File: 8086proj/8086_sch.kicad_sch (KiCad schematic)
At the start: 1 part, among them U1 8086_Min_Mode

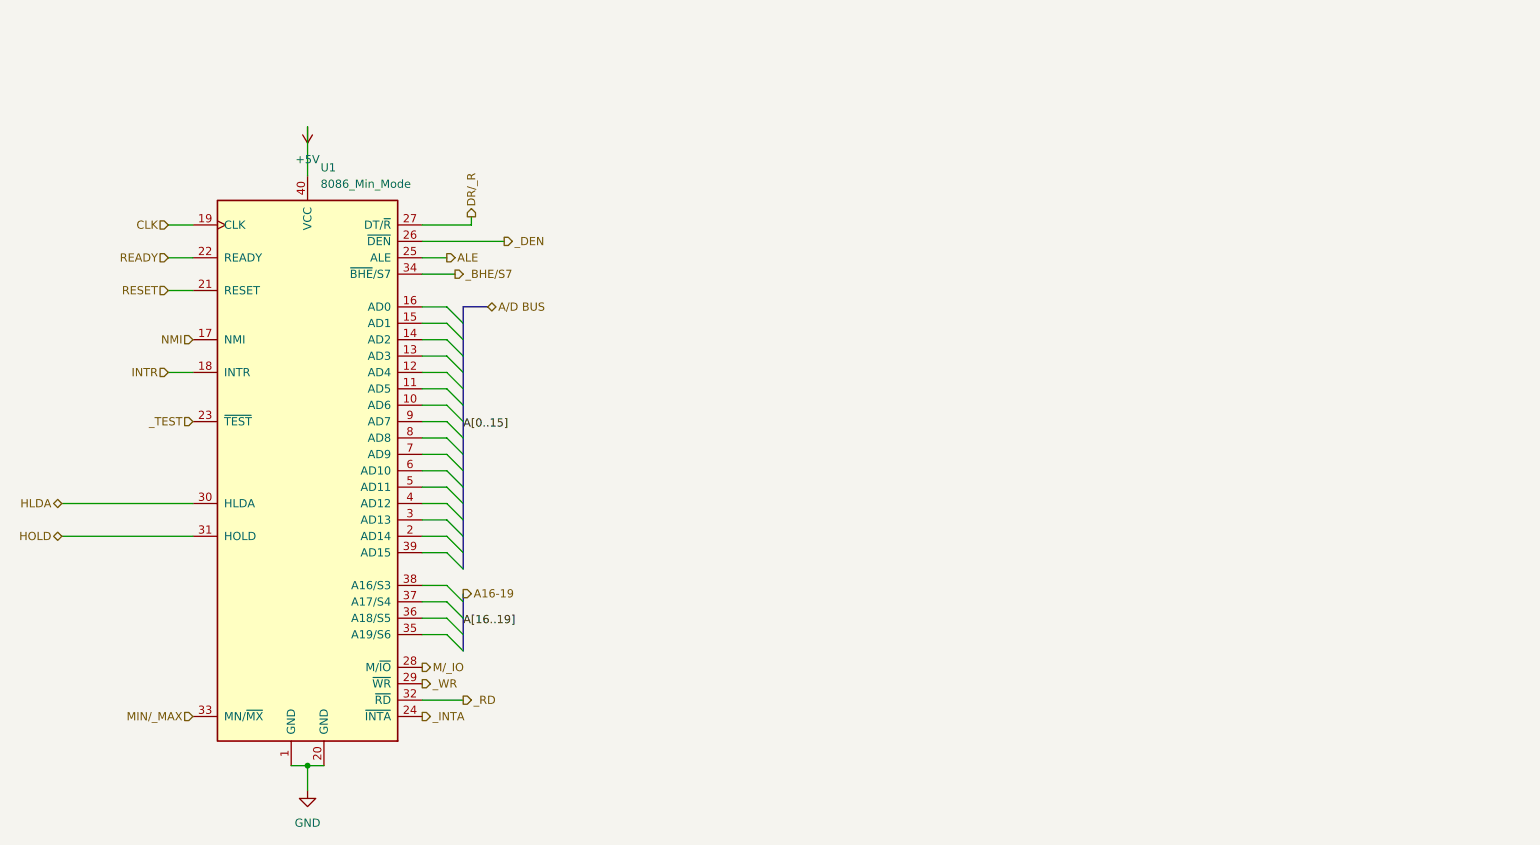
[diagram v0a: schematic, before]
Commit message: latch added
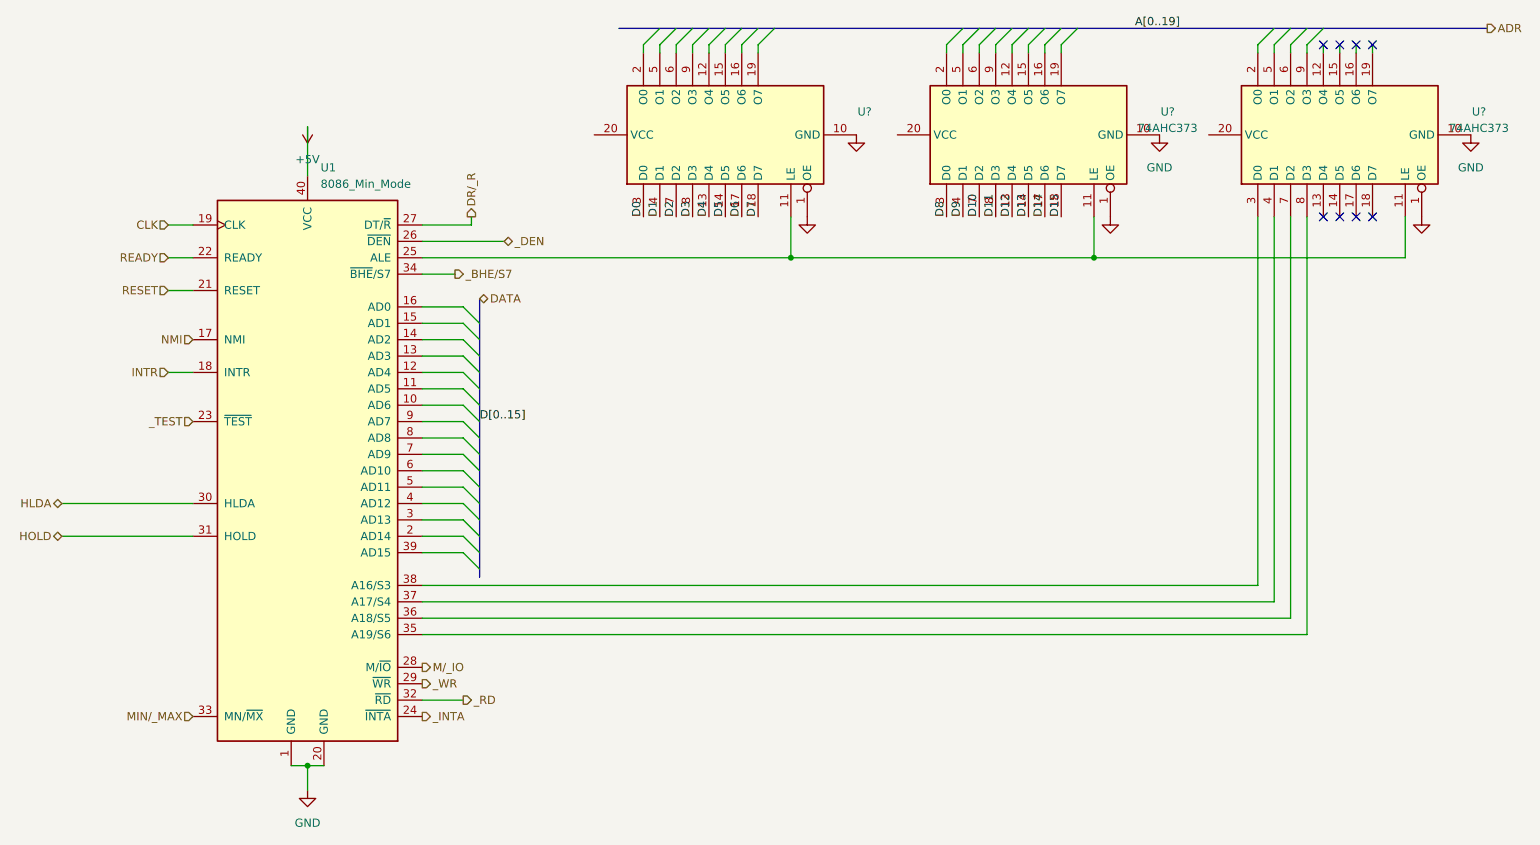
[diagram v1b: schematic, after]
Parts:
- added U? (x2): 74AHC373, symbol 74xx:74AHC373
- added U?: (no value), symbol 74xx:74AHC373
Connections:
- net GND: now also U?.1 (OE), U?.1 (OE), U?.1 (OE), U?.10 (GND), U?.10 (GND), U?.10 (GND)
- net at U1.35 (A19/S6): now also U?.8 (D3)
- net at U1.36 (A18/S5): now also U?.7 (D2)
- net at U1.37 (A17/S4): now also U?.4 (D1)
- net at U1.38 (A16/S3): now also U?.3 (D0)
- net ALE: no longer names the net of U1.25 (ALE)
- net ALE: now also U?.11 (LE), U?.11 (LE), U?.11 (LE)
- new net D0: U?.3 (D0)
- new net D1: U?.4 (D1)
- new net D10: U?.7 (D2)
- new net D11: U?.8 (D3)
- new net D12: U?.13 (D4)
- new net D13: U?.14 (D5)
- new net D14: U?.17 (D6)
- new net D15: U?.18 (D7)
- new net D2: U?.7 (D2)
- new net D3: U?.8 (D3)
- new net D4: U?.13 (D4)
- new net D5: U?.14 (D5)
- new net D6: U?.17 (D6)
- new net D7: U?.18 (D7)
- new net D8: U?.3 (D0)
- new net D9: U?.4 (D1)
- no-connect marks 0 -> 8
